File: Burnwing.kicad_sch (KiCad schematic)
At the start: 41 parts, among them J1 USB Type C, J2 Conn_01x06_MountingPin, J3 Conn_01x02_Pin, Q1 NCV8402ADDR2G, Q2 AONR21307, U1 HUSB238

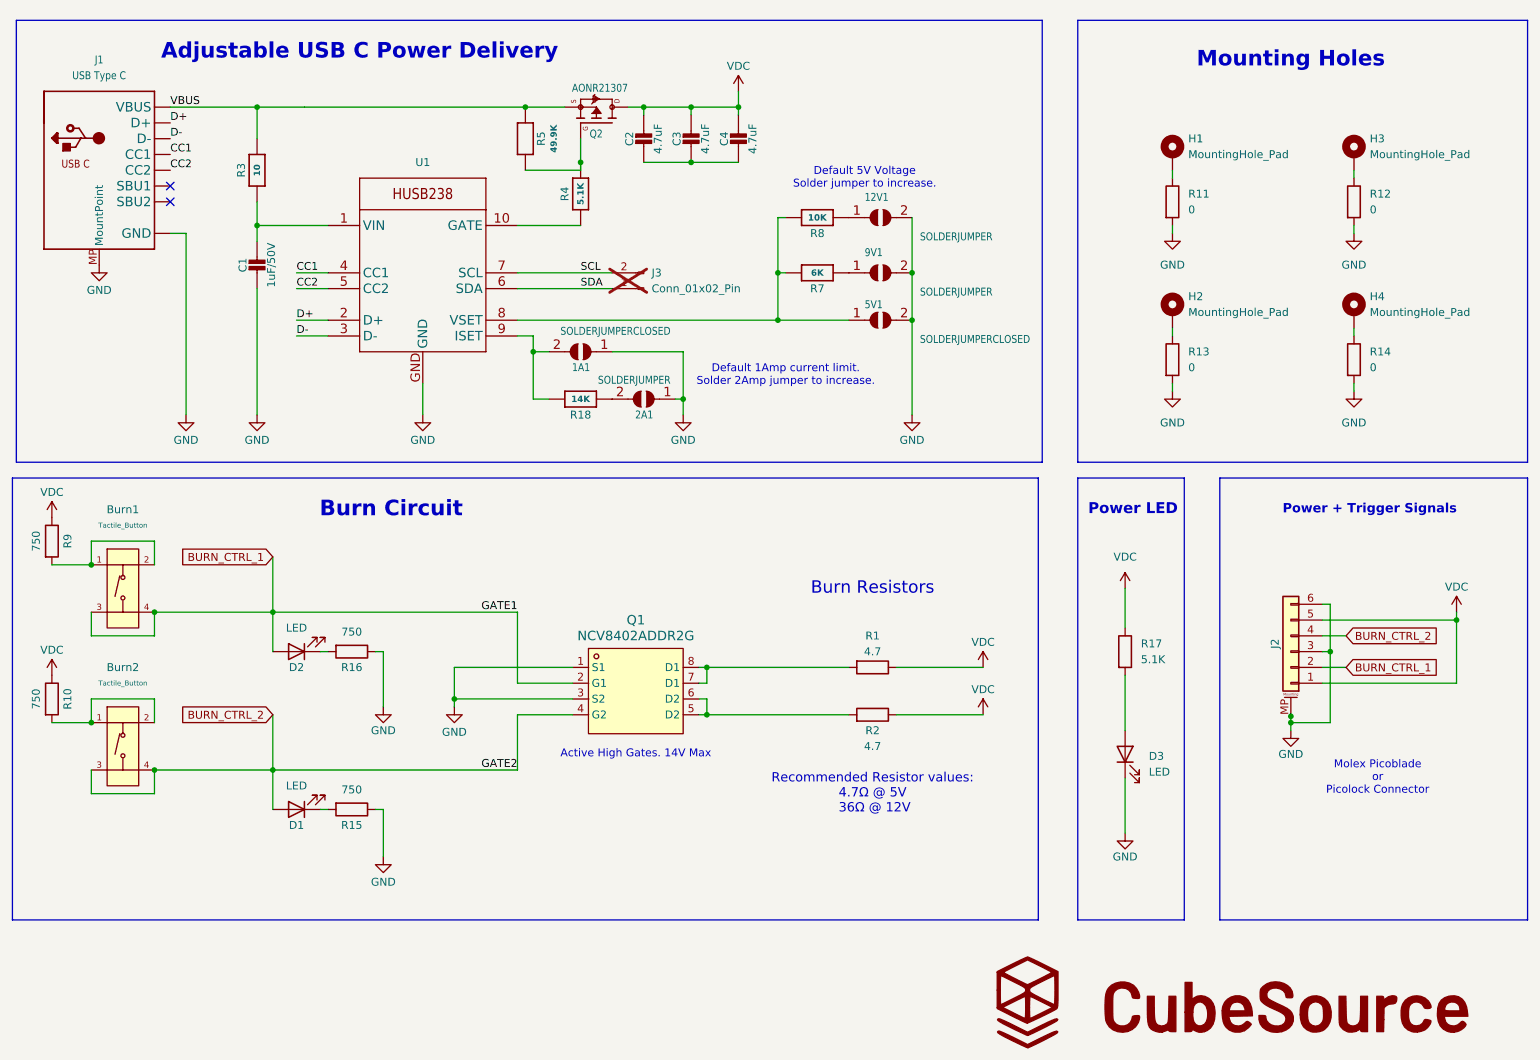
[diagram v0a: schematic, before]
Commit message: Cleaned schematic a bit
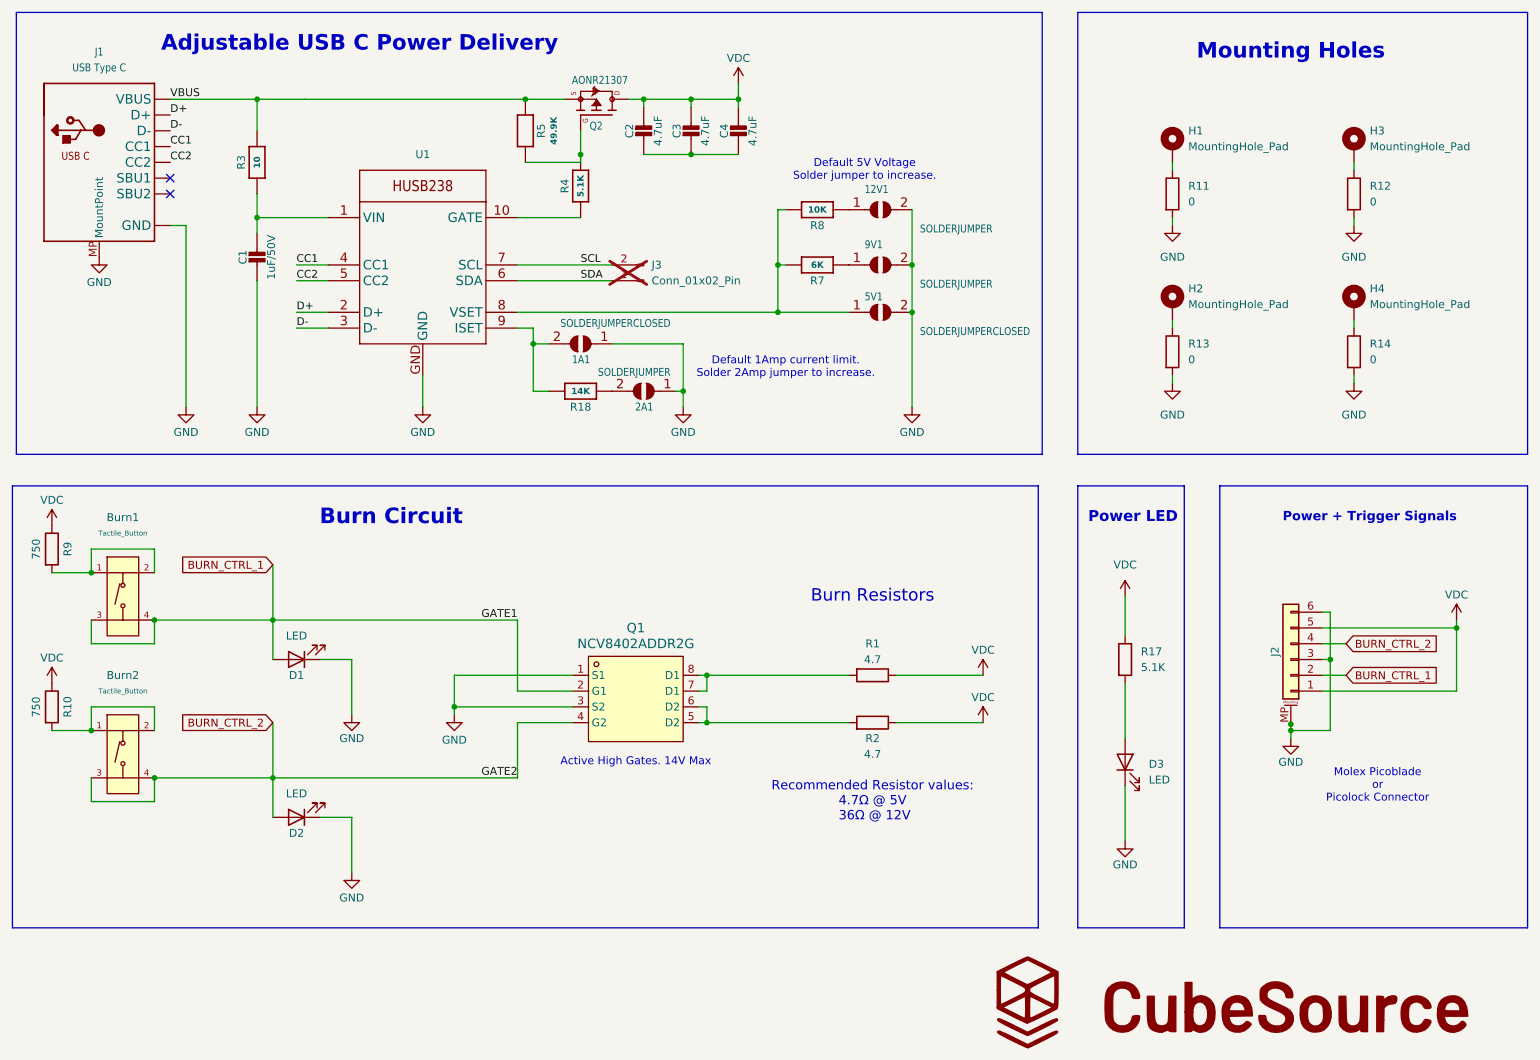
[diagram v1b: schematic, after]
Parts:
- removed R15, R16: 750, Resistor_SMD:R_0603_1608Metric_Pad0.98x0.95mm_HandSolder, symbol Library:R
- renumbered D2 to D1, D1 to D2
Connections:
- net GND: now also D1.1 (K), D2.1 (K)
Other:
- moved on the sheet: 12V1, 1A1, 2A1, 5V1, 9V1, Burn1, Burn2, C1, C2, C3, C4, D1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
